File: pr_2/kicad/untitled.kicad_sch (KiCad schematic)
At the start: 1 part, among them SW1 RotaryEncoder_Switch

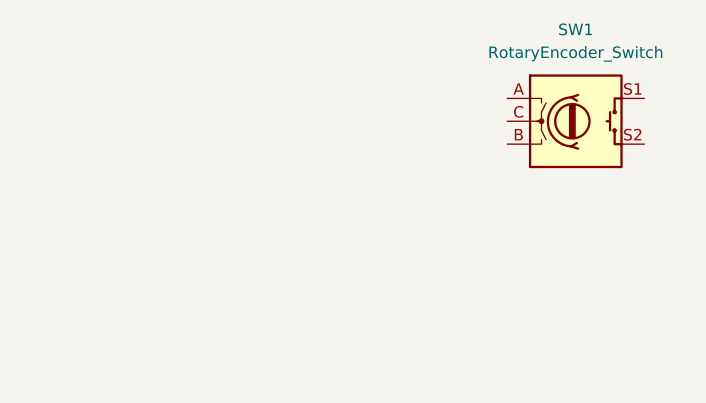
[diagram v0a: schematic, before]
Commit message: feat: added kicad schema
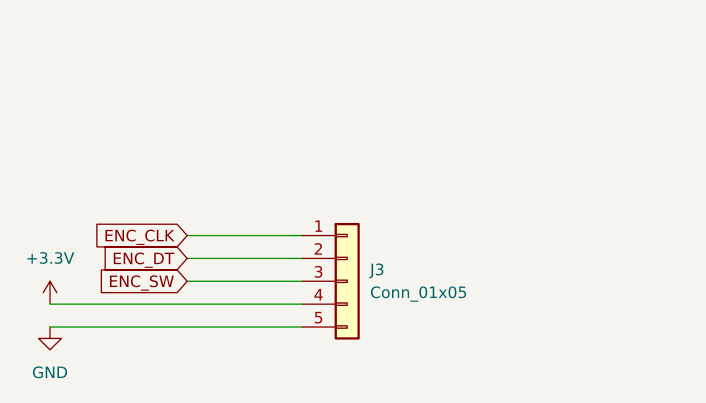
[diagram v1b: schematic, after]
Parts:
- removed SW1: RotaryEncoder_Switch, symbol Device:RotaryEncoder_Switch
- added J3: Conn_01x05, symbol Connector_Generic:Conn_01x05
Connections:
- new net +3.3V: J3.4 (Pin_4)
- new net ENC_CLK: J3.1 (Pin_1)
- new net ENC_DT: J3.2 (Pin_2)
- new net ENC_SW: J3.3 (Pin_3)
- new net GND: J3.5 (Pin_5)
